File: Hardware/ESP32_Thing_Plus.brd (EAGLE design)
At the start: 33 x 58.9 mm, 54 parts, among them Q1 2.5A/30V, Q2 MBT3904DW1T1, U1 MCP73831, U2 ESP-WROOM-32, U3 AP2112K-3.3V, U4 FT231XS

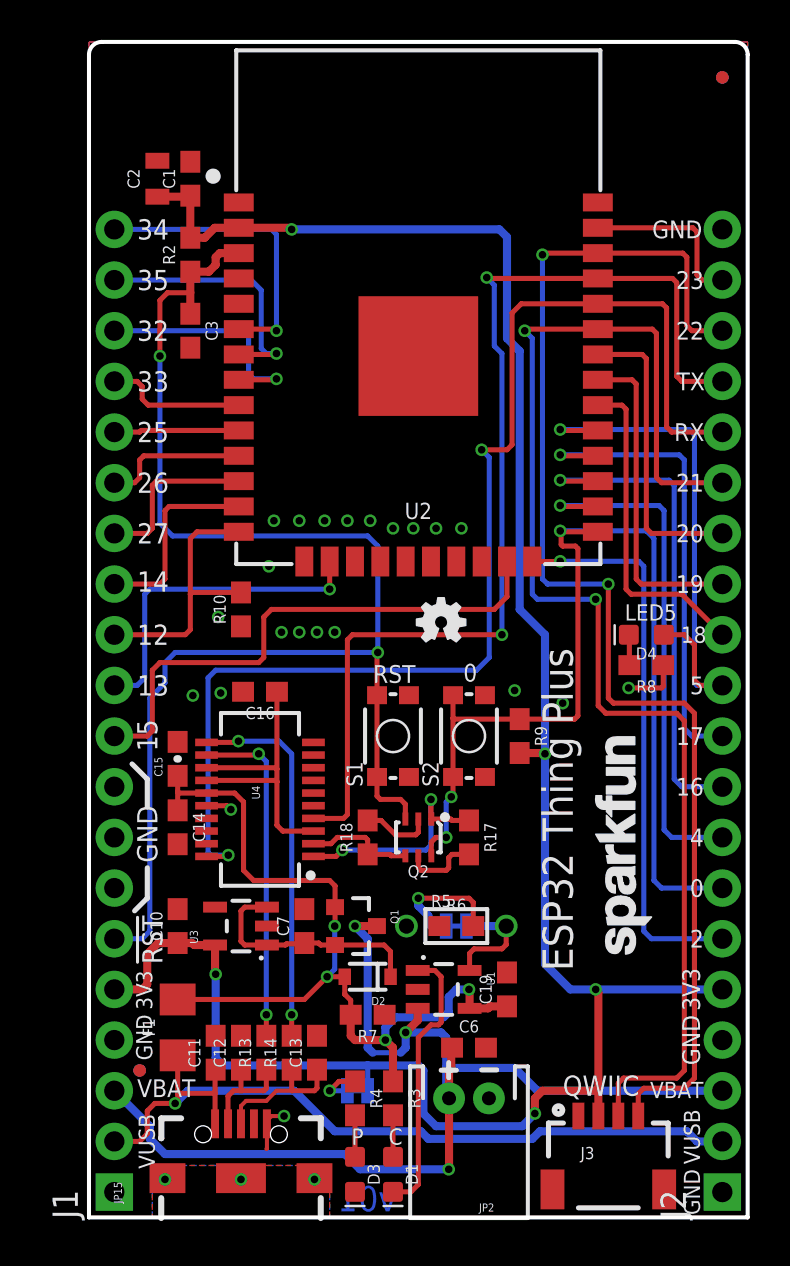
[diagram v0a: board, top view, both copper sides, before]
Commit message: Feedback from review
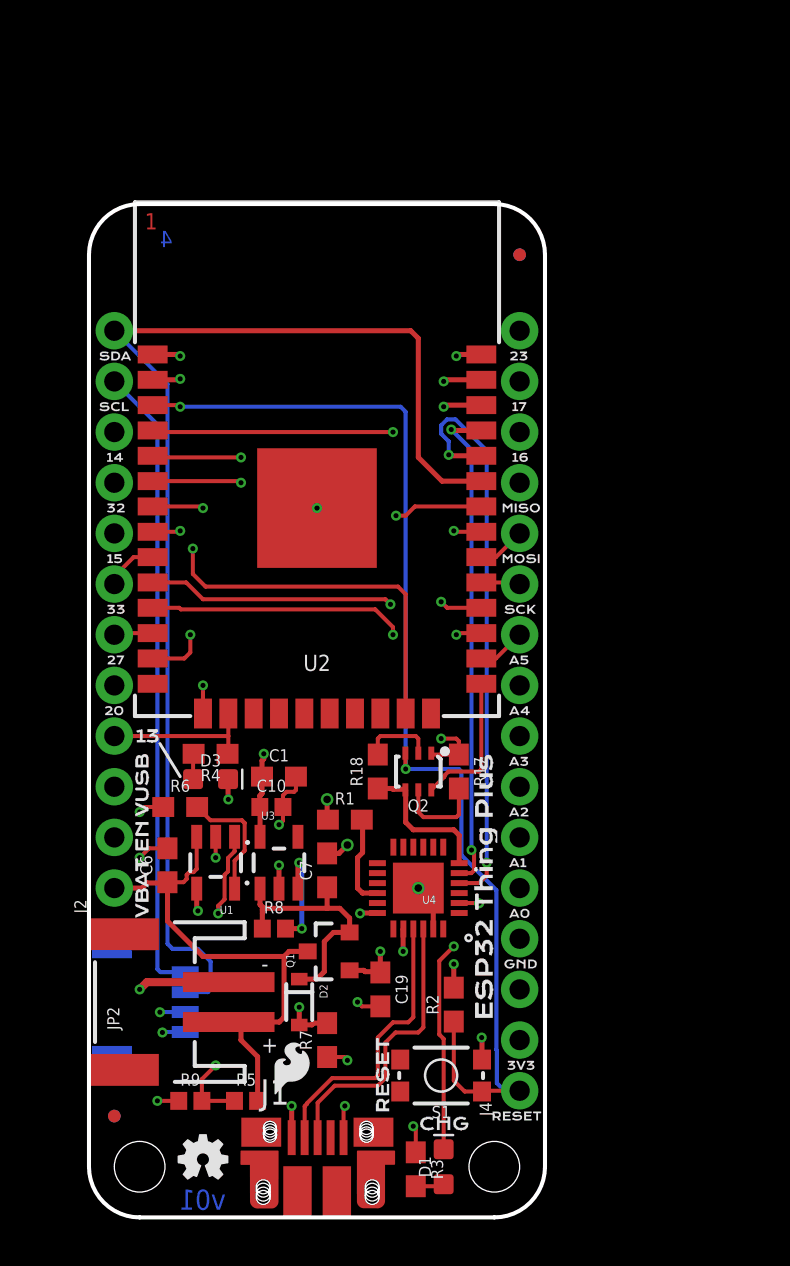
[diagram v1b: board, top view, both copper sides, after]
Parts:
- removed C11, C14, C16, C3: 0.1uF, SparkFun-Capacitors:0603
- removed C12, C13: 47pF, SparkFun-Capacitors:0603
- removed C15: 4.7uF, SparkFun-Capacitors:0603-CAP
- removed C2: 10uF, SparkFun-Capacitors:0805
- removed D4: BLUE, SparkFun-LED:LED-0603
- removed F1: 6V/0.75A, SparkFun-Fuses:1206
- removed JP15: (no value), SparkFun-Connectors:USB-B-MICRO-SMD_V03
- removed R10: 10k, SparkFun-Resistors:0603
- removed R13, R14: 27, SparkFun-Resistors:0603
- removed S2: BTN-0, SparkFun-Electromechanical:TACTILE_SWITCH_SMD_4.6X2.8MM
- removed SJ1, SJ2: JUMPER-PAD-2-NC_BY_TRACE, SparkFun-Passives:PAD-JUMPER-2-NC_BY_TRACE_YES_SILK
- added J4: (no value), SparkFun-Connectors:1X16_NO_SILK
- added LOGO4: FOUR_LAYER_WARNING, SparkFun-Aesthetics:FOUR_LAYER_WARNING
- added R1: 1k, SparkFun-Resistors:0603
- added U$1: (no value), buzzard_labels:3V322
- added U$10: (no value), buzzard_labels:1611
- added U$11: (no value), buzzard_labels:1710
- added U$12: (no value), buzzard_labels:A020
- added U$13: (no value), buzzard_labels:A119
- added U$14: (no value), buzzard_labels:A218
- added U$15: (no value), buzzard_labels:A317
- added U$16: (no value), buzzard_labels:A416
- added U$17: (no value), buzzard_labels:A515
- added U$18: (no value), buzzard_labels:GND21
- added U$19: (no value), buzzard_labels:MISO12
- added U$2: (no value), buzzard_labels:138
- added U$20: (no value), buzzard_labels:MOSI13
- added U$21: (no value), buzzard_labels:SCK14
- added U$22: (no value), buzzard_labels:RESET23
- added U$23: (no value), buzzard_labels:SCL1
- added U$24: (no value), buzzard_labels:SDA0
- added U$25: (no value), buzzard_labels (1):CHG3
- added U$26: (no value), buzzard_labels (1):EN1
- added U$27, U$30: (no value), buzzard_labels (1):ESP32_THING_PLUS4
- added U$28: (no value), buzzard_labels (1):VBAT2
- added U$29: (no value), buzzard_labels (1):VUSB0
- added U$3: (no value), buzzard_labels:142
- added U$31: (no value), buzzard_labels (2):3V313
- added U$32: (no value), buzzard_labels (2):#RESET17
- added U$33: (no value), buzzard_labels (2):162
- added U$34: (no value), buzzard_labels (2):171
- added U$35: (no value), buzzard_labels (2):230
- added U$36: (no value), buzzard_labels (2):1326
- added U$37: (no value), buzzard_labels (2):1420
- added U$38: (no value), buzzard_labels (2):1522
- added U$39: (no value), buzzard_labels (2):2025
- added U$4: (no value), buzzard_labels:154
- added U$40: (no value), buzzard_labels (2):2724
- added U$41: (no value), buzzard_labels (2):3221
- added U$42: (no value), buzzard_labels (2):3323
- added U$43: (no value), buzzard_labels (2):A011
- added U$44: (no value), buzzard_labels (2):A29
- added U$45: (no value), buzzard_labels (2):A38
- added U$46: (no value), buzzard_labels (2):A47
- added U$47: (no value), buzzard_labels (2):A56
- added U$48: (no value), buzzard_labels (2):A110
- added U$49: (no value), buzzard_labels (2):EN16
- added U$5: (no value), buzzard_labels:207
- added U$50: (no value), buzzard_labels (2):GND12
- added U$51: (no value), buzzard_labels (2):MISO3
- added U$52: (no value), buzzard_labels (2):MOSI4
- added U$53: (no value), buzzard_labels (2):SCK5
- added U$54: (no value), buzzard_labels (2):SCL19
- added U$55: (no value), buzzard_labels (2):SDA18
- added U$56: (no value), buzzard_labels (2):VBAT15
- added U$57: (no value), buzzard_labels (2):VUSB14
- added U$58: (no value), buzzard_labels (3):QWIIC0
- added U$59: (no value), SparkFun-Aesthetics:ORDERING_INSTRUCTIONS
- added U$6: (no value), buzzard_labels:239
- added U$60: (no value), buzzard_labels (5):RESET0
- added U$7: (no value), buzzard_labels:276
- added U$8: (no value), buzzard_labels:323
- added U$9: (no value), buzzard_labels:335
- C1: value 0.1uF -> 10uF
- C10: value 2.2uF -> 1.0uF; device SparkFun-Capacitors:0603 -> SparkFun-Capacitors:0402
- D3: value RED -> BLUE
- FD1, FD2, FD3, FD4: device SparkFun-Aesthetics:MICRO-FIDUCIAL -> SparkFun-Aesthetics:FIDUCIAL-MICRO
- J1: value (none) -> AMP FCI 10103594-0001LF; device SparkFun-Connectors:1X20_NOSILK -> SparkFun-Connectors:USB-MICROB-PTH
- J2: device SparkFun-Connectors:1X20_NOSILK -> SparkFun-Connectors:1X12_NO_SILK
- JP2: device SparkFun-Connectors:JST-2-PTH -> SparkFun-Connectors:JST-2-SMD
- LOGO1: value SFE_LOGO_NAME.1_INCH -> SFE_LOGO_FLAME.1_INCH; device SparkFun-Aesthetics:SFE_LOGO_NAME_.1 -> SparkFun-Aesthetics:SFE_LOGO_FLAME_.1
- LOGO3: value SFE_LOGO_NAME.2_INCH -> SFE_LOGO_NAME_FLAME.1_INCH; device SparkFun-Aesthetics:SFE_LOGO_NAME_.2 -> SparkFun-Aesthetics:SFE_LOGO_NAME_FLAME_.1
- R4: value 1K -> 1k
- R5: value DNP -> 100K; device SparkFun-Passives:1/6W-RES -> SparkFun-Resistors:0402
- R8: value 330 -> 100K; device SparkFun-Resistors:0603 -> SparkFun-Resistors:0402
- R9: value 10k -> 100K; device SparkFun-Resistors:0603 -> SparkFun-Resistors:0402
- S1: device SparkFun-Electromechanical:TACTILE_SWITCH_SMD_4.6X2.8MM -> SparkFun-Switches:TACTILE_SWITCH_SMD_4.6X2.8MM
- U2: value ESP-WROOM-32 -> ESP-WROOM-32NARROW; device SparkFun-RF:ESP-WROOM-32 -> SparkFun-RF:ESP-WROOM-32-NARROW
- U4: value FT231XS -> CP2102N; device SparkFun-DigitalIC:SSOP20_L -> SparkFun-IC-Comms:QFN24
- moved FD4 60.3 mm to (1.27, 5.08)
- moved FD1 45.1 mm to (21.6, 48.3)
- moved R2 39.8 mm to (18.3, 10.7)
- moved J2 34.1 mm to (1.27, 16.5)
- moved C1 30.3 mm to (9.53, 22.1), turned to 0 degrees
- moved LOGO2 29.5 mm to (5.71, 2.92)
- moved R9 24.6 mm to (5.08, 5.84), turned to 0 degrees
- moved R8 22.9 mm to (9.27, 14.5), turned to 0 degrees
- moved J3 22.0 mm to (4.83, 10.8), flipped to the bottom, turned to 90 degrees
- moved D3 21.1 mm to (6.10, 22.0), turned to 0 degrees
- moved LOGO1 20.8 mm to (9.02, 5.84), turned to 0 degrees
- moved R4 18.7 mm to (6.10, 23.2), turned to 180 degrees
- moved C6 17.7 mm to (3.94, 17.7), turned to 90 degrees
- moved S1 17.2 mm to (17.7, 7.11), turned to 180 degrees
- moved JP2 16.5 mm to (3.30, 10.8), turned to 90 degrees
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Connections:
- net N$9 renamed CHG
- removed net 18: J2.12, U2.30
- removed net 19: J2.13, U2.31
- removed net 21: J2.15, J3.3, U2.33
- removed net 22: J2.18, J3.4, U2.36
- removed net 25: J1.16, U2.10
- removed net 26: J1.15, U2.11
- removed net 3.3V_F: C16.1, U4.13, U4.14, U4.3
- removed net 34: J1.20, U2.6
- removed net 4: J2.8, U2.26
- removed net 5: D4.A, J2.11, U2.29
- removed net N$16: R6.2, SJ1.1
- removed net N$3: R4.1, SJ2.1
- removed net N$7: R13.2, U4.12
- removed net N$8: R14.2, U4.11
- removed net SHIELD: JP15.SHIELD1, JP15.SHIELD2, JP15.SHIELD3
- removed net U0RXD: J2.16, U2.34, U4.20
- removed net U0TXD: J2.17, U2.35, U4.4
- removed net VUSB-RAW: C11.1, F1.1, J1.2, J2.2, JP15.VBUS
- new net A0: J4.5, U2.11
- new net A1: J4.6, U2.10
- new net A2: J4.7, U2.6
- new net A3: J4.8, U2.5
- new net A4: J4.9, U2.4
- new net A5: J4.10, U2.26
- new net EN: J2.2, R8.2, U3.3
- new net MISO: J4.13, U2.31
- new net MOSI: J4.12, U2.30
- new net RX: U2.35, U4.20
- new net SCK: J4.11, U2.29
- new net SCL: J2.11, J3.4, U2.36
- new net SDA: J2.12, J3.3, U2.33
- new net TX: U2.34, U4.21
- new net VDD: U4.6
- net 0: no longer J2.7, R9.1, S2.3, S2.4
- net 12: no longer J1.12, R10.2
- net 13: now also J2.4, R4.1; no longer J1.11
- net 14: now also J2.10; no longer J1.13
- net 15: now also J2.8; no longer J1.10
- net 16: now also J4.14; no longer J2.9
- net 17: now also J4.15; no longer J2.10
- net 2: no longer J2.6
- net 20: now also J2.5; no longer J2.14
- net 23: now also J4.16; no longer J2.19
- net 27: now also J2.6; no longer J1.14
- net 3.3V: now also J4.2, R1.1, U4.5; no longer C2.1, J1.5, J2.5, R9.2, SJ2.2
- net 32: now also J2.9; no longer J1.18
- net 33: now also J2.7; no longer J1.17
- net 35: now also R5.1, R9.2; no longer J1.19
- net CHIP_PU: now also J4.1; no longer C3.1, J1.6, S1.3
- net D+: now also J1.D+, U4.3; no longer C13.1, JP15.D+, R14.1
- net D-: now also J1.D-, U4.4; no longer C12.1, JP15.D-, R13.1
- net DTR: now also U4.23; no longer U4.1
- net GND: now also J1.GND, J4.4, JP2.2, R9.1, U4.2, U4.PAD; no longer C11.2, C12.2, C13.2, C14.2, C15.2, C16.2, C2.2, C3.2, J1.1, J1.4, J1.7, J1.8, J1.9, J2.1, J2.20, J2.4, JP15.GND, JP2.1, R10.1, R5.1, R8.1, S1.2, S2.1, S2.2, U4.16, U4.6
- net N$1: now also R1.2, U4.9; no longer D4.C, R8.2
- net N$14: now also R6.2; no longer R5.2, SJ1.2
- net RTS: now also U4.19; no longer U4.2
- net VIN: now also R8.1; no longer U3.3
- net V_BATT: now also J2.1, JP2.1, R5.2; no longer J1.3, J2.3, JP2.2
- net V_USB: now also J1.VBUS, J2.3, U4.7; no longer C14.1, C15.1, F1.2, U4.15
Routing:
- net 3.3V: track 111.3 -> 26.5 mm, vias 5 -> 6
- net 21: track 66.8 -> 0.00 mm, vias 2 -> 0
- net 22: track 65.2 -> 0.00 mm, vias 2 -> 0
- net SDA: track 0.00 -> 62.1 mm
- net U0RXD: track 61.2 -> 0.00 mm, vias 2 -> 0
- net U0TXD: track 53.3 -> 0.00 mm, vias 2 -> 0
- net SCL: track 0.00 -> 51.1 mm, vias 0 -> 1
- net 0: track 52.6 -> 7.26 mm, vias 3 -> 0
- net VUSB-RAW: track 40.6 -> 0.00 mm, vias 1 -> 0
- net V_USB: track 43.2 -> 9.94 mm, vias 4 -> 6
- net A2: track 0.00 -> 30.7 mm, vias 0 -> 1
- net A3: track 0.00 -> 30.4 mm, vias 0 -> 1
- net V_BATT: track 56.3 -> 26.3 mm, vias 3 -> 0
- net A4: track 0.00 -> 29.8 mm, vias 0 -> 1
- net TX: track 0.00 -> 29.2 mm, vias 0 -> 2
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- added copper zone on layer 15, net 3.3V
- added copper zone on layer 2, net GND
- added copper zone on layer 15, net V_USB
- removed copper zone on layer 1, net GND
- removed copper zone on layer 16, net GND
- removed copper zone on layer 1, net SHIELD
- removed copper zone on layer 16, net SHIELD
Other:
- board size 33 x 58.9 mm -> 22.9 x 50.8 mm
- board text added: "+"
- board text added: "-"
- board text added: "1"
- board text added: "3"
- board text removed: "!RST"
- board text removed: "0"
- board text removed: "12"
- board text removed: "13"
- board text removed: "14"
- board text removed: "15"
- board text removed: "16"
- board text removed: "17"
- board text removed: "18"
- board text removed: "19"
- board text removed: "20"
- board text removed: "21"
- board text removed: "22"
- board text removed: "23"
- board text removed: "25"
- board text removed: "26"
- board text removed: "27"
- board text removed: "32"
- board text removed: "33"
- board text removed: "34"
- board text removed: "35"
- board text removed: "3V3"
- board text removed: "5"
- board text removed: "C"
- board text removed: "CHG PROG"
- board text removed: "ESP32 Thing Plus"
- board text removed: "GND"
- board text removed: "LED5"
- board text removed: "Measurements in inches"
- board text removed: "P"
- board text removed: "PWR LED"
- board text removed: "QWIIC"
- board text removed: "RST"
- board text removed: "RX"
- board text removed: "RXI"
- board text removed: "TX"
- board text removed: "TXO"
- board text removed: "VBAT"
- board text removed: "VUSB"
